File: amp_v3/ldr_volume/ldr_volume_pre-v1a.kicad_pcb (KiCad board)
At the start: 2 copper layers, 316.9 x 199.6 mm, 163 parts, among them J1 PWR1, J10 5v_in, J11 CTRL, J12 I2C_R, J13 A_IN, J14 A_OUT, J15 ADS1115, J16 MUTE_OUT, J17 MUTE, J18 UART, J19 MUTE, J2 PWR2, J20 CTRL, J21 CTRL, J22 PWR_IN, J23 I2C_L, J24 I2C_R, J26 TFT, J27 PWR_BTN, J28 PWR_BTN_LED, J29 PWR_IN, J3 PWR3, J30 I2C, J31 BTN_VOL, J32 BTN_MENU, J33 ALPS, J34 PWR_RLY, J35 BTN_EXT1, J36 BTN_EXT2, J38 IR, J39 MUTE, J4 PWR4, J40 UART, J41 IR_SENSOR, J42 S_AIN_L, J43 S_AIN_R, J5 PWR3, J6 PWR4, J7 Conn_01x03_Pin, J8 5V_IN, J9 5V_IN, K1 G5V-2, Q1 BC557, Q10 2N7000, Q11 BC547, Q12 BC547, Q2 BC557, Q3 BC547, Q4 BC547, Q5 BC557, Q6 BC557, Q7 BC547, Q8 BC547, Q9 2N7000, SW1 SW_LT, SW2 SW_RT, SW3 SW_UP, SW4 SW_DN, SW5 SW_PWR, U1 IRM-10-5, U2 NSL-32-SR3-Rseries, U3 MCP1700x-330xxTO, U4 NSL-32-SR3-Rshunt, U5 4N25, U6 TSOP312xx

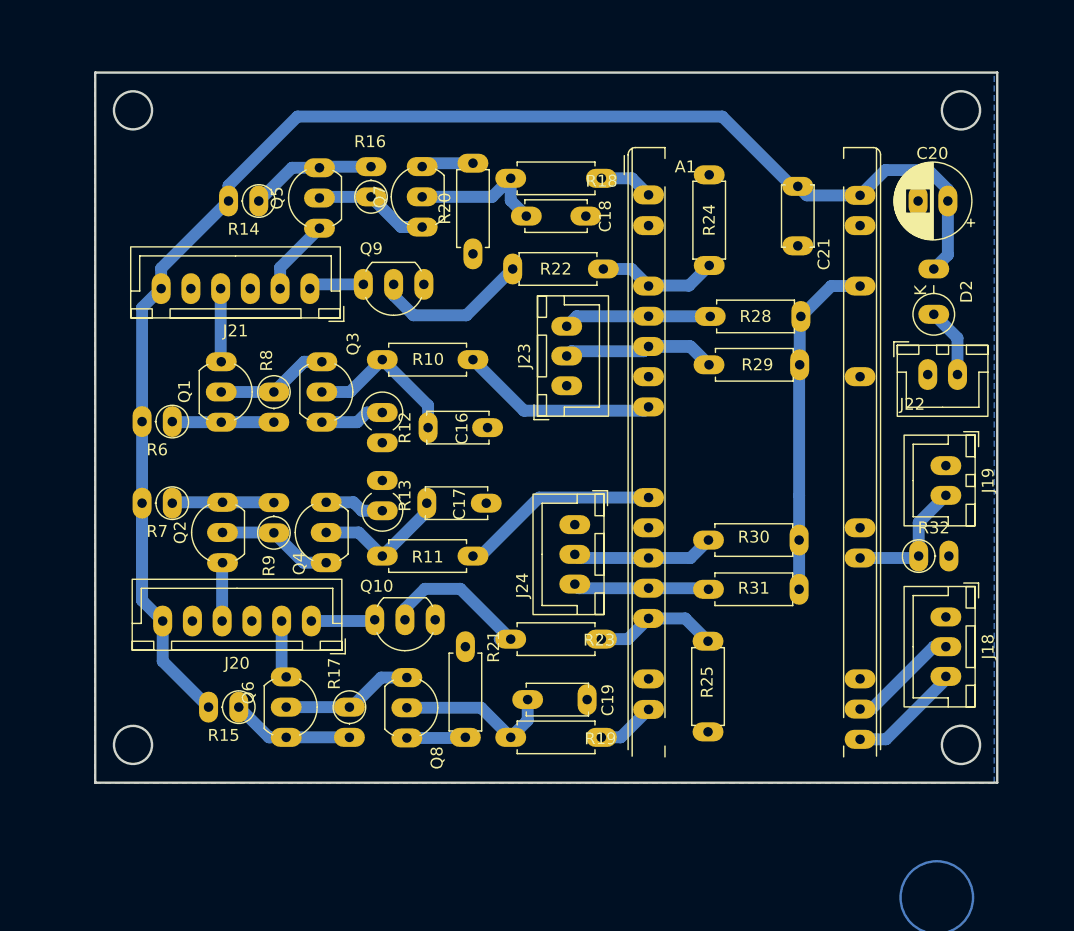
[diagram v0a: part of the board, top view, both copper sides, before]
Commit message: updates
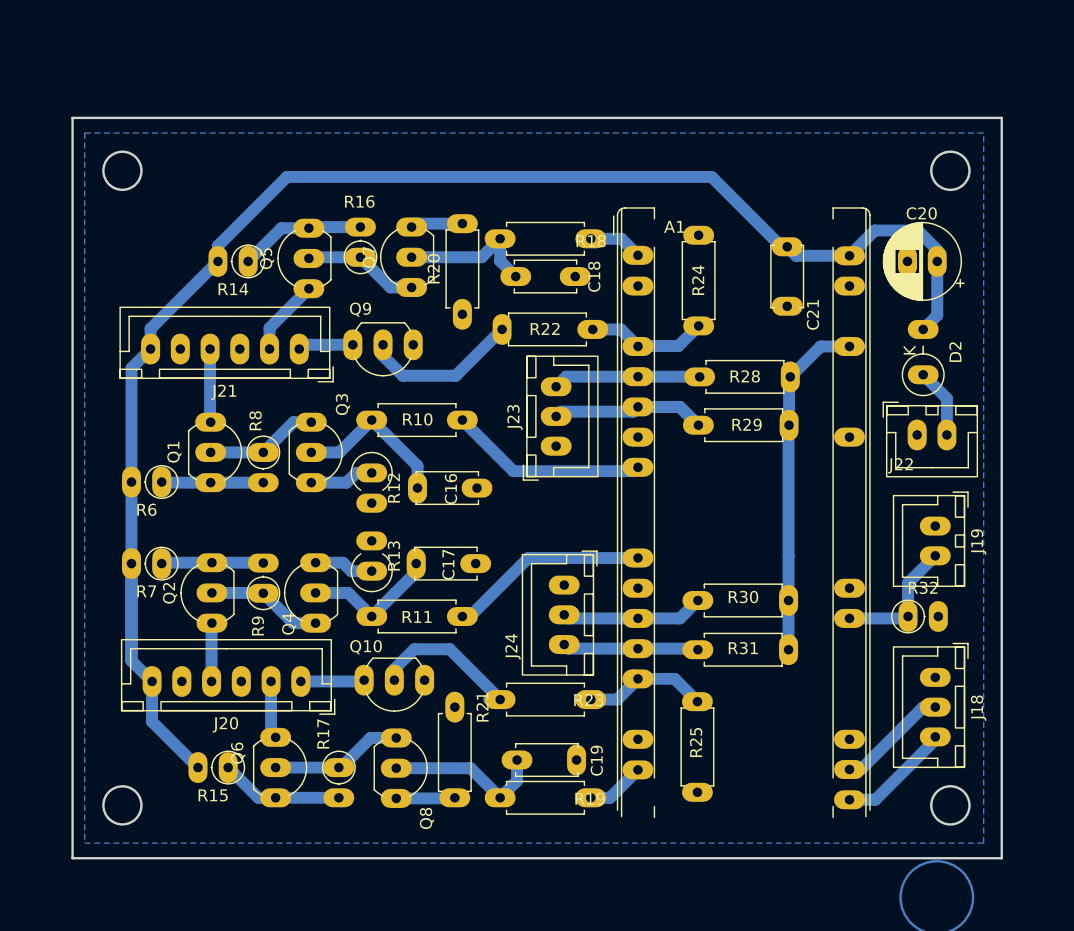
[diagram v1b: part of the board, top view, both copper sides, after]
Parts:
- moved C20 5.16 mm to (146.3, -155.0)
- moved C21 5.16 mm to (133.6, -156.2)
- moved D2 5.16 mm to (145.1, -149.3)
- moved J19 5.16 mm to (146.1, -132.7)
- moved Q2 5.16 mm to (85.3, -124.6)
- moved Q3 5.16 mm to (93.6, -141.5)
- moved Q4 5.16 mm to (94.0, -124.6)
- moved R10 5.16 mm to (98.7, -141.6)
- moved R11 5.16 mm to (98.7, -125.1)
- moved R12 5.16 mm to (98.7, -137.2)
- moved R13 5.16 mm to (98.7, -128.9)
- moved R18 5.16 mm to (109.5, -156.9)
- moved R30 5.16 mm to (133.8, -126.5)
- moved R32 5.16 mm to (143.8, -125.1)
- moved R8 5.16 mm to (89.6, -138.9)
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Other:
- outline, holes or cut-outs redrawn
